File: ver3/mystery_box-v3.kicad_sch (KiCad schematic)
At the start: 31 parts, among them J10 Screw_Terminal_01x02, J11 Screw_Terminal_01x02, J12 Screw_Terminal_01x02, J13 Screw_Terminal_01x02, J14 Screw_Terminal_01x02, J15 Screw_Terminal_01x02, J16 Screw_Terminal_01x02, J17 Screw_Terminal_01x02, J18 Barrel_Jack_MountingPin, J20 rj45-CC-X2-Aliexpress, J8 Screw_Terminal_01x02, J9 Screw_Terminal_01x02, Q1 IRLZ44N, Q2 IRLZ44N, Q3 IRLZ44N, U2 MAX485E

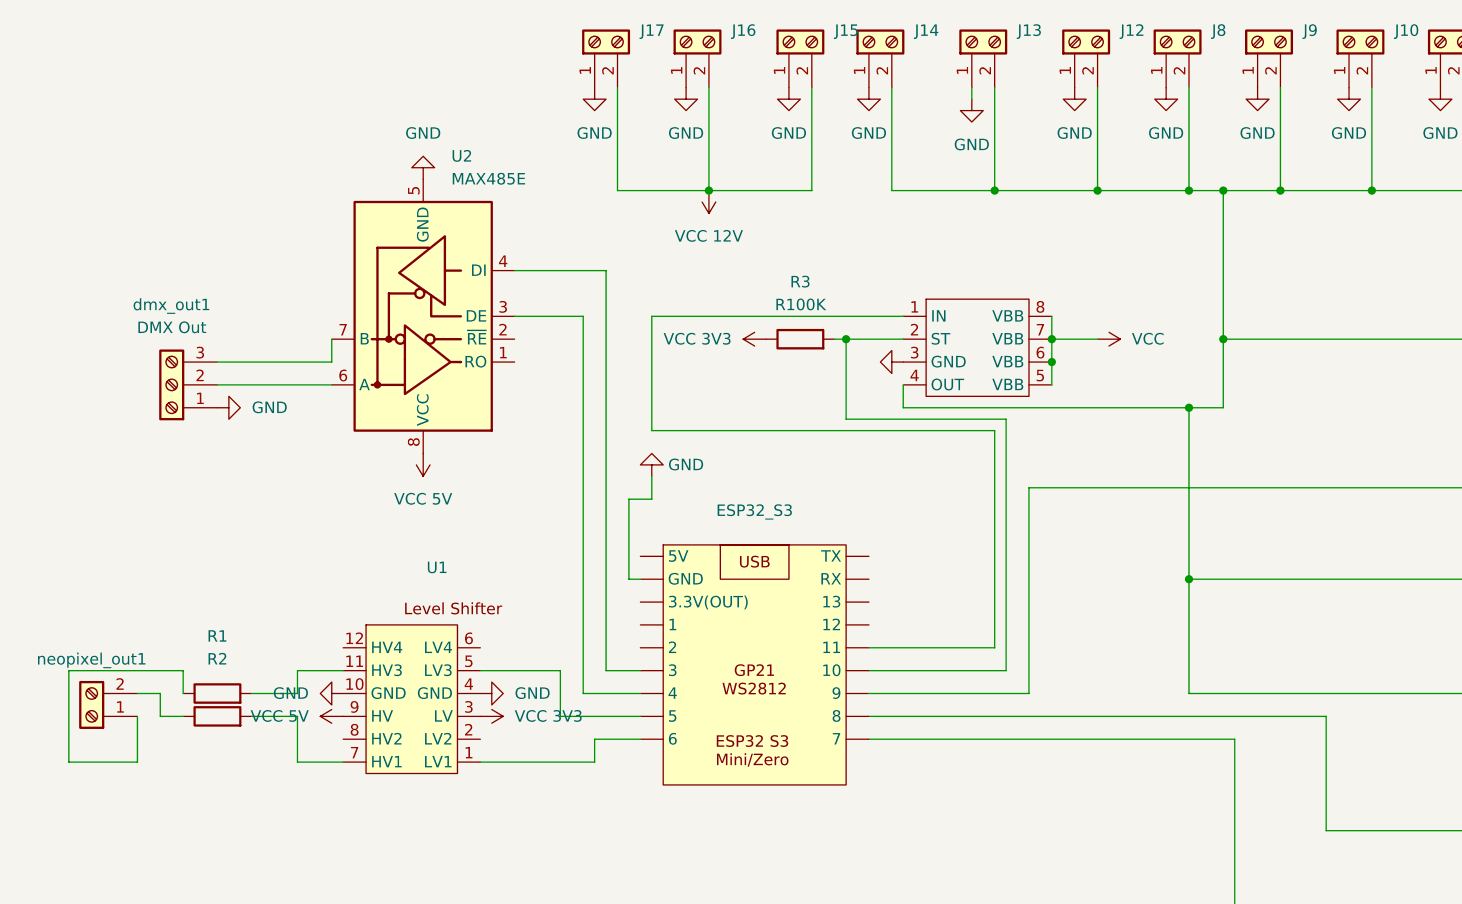
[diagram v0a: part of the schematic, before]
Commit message: final prototype v3
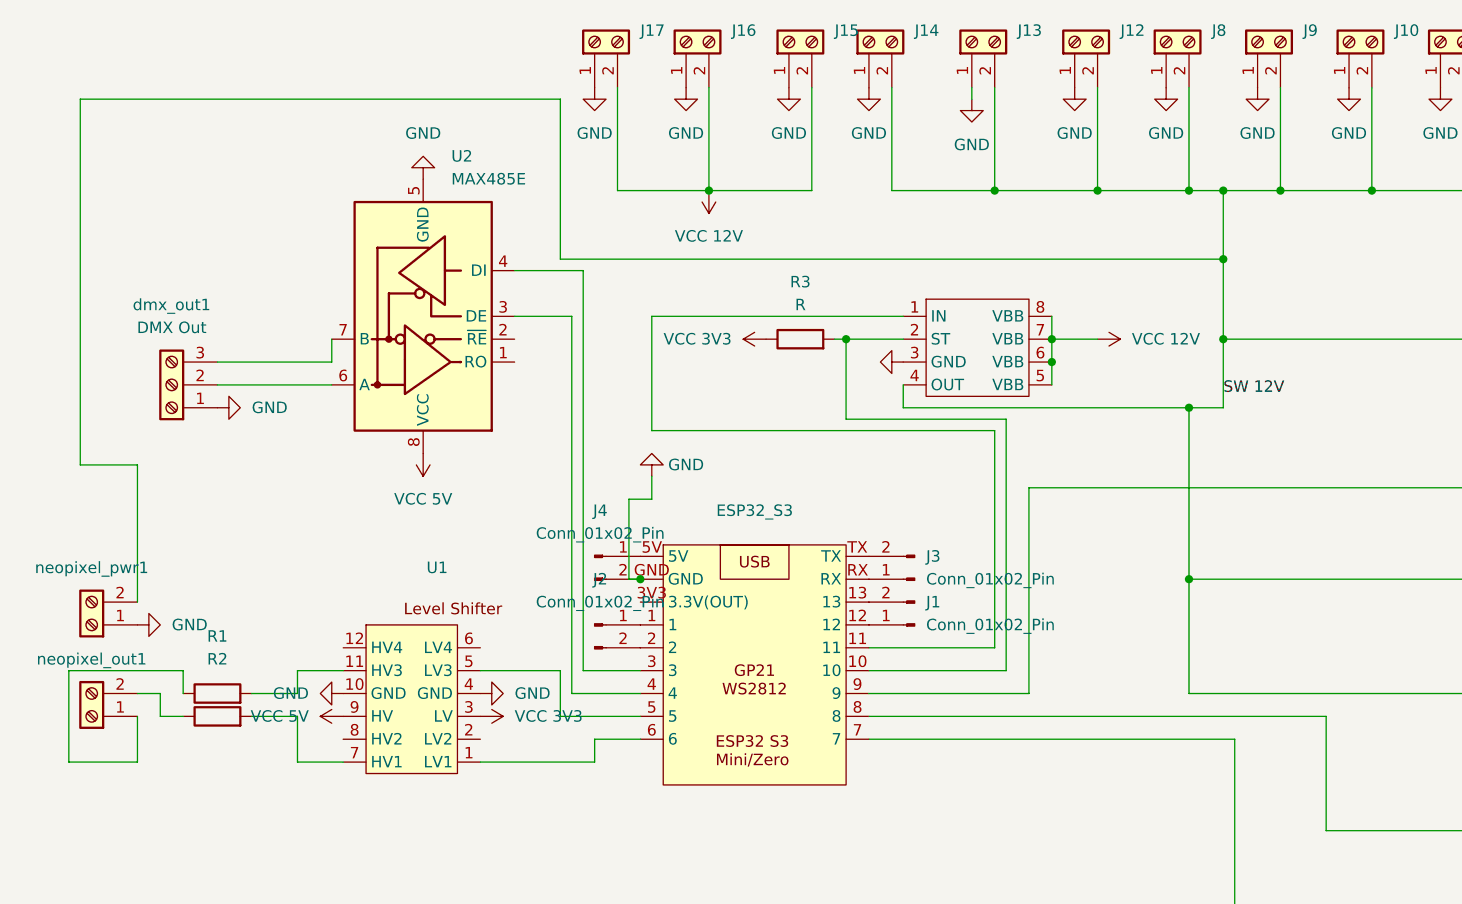
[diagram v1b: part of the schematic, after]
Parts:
- added J1, J2, J3, J4: Conn_01x02_Pin, Connector_PinHeader_1.00mm:PinHeader_1x02_P1.00mm_Vertical, symbol Connector:Conn_01x02_Pin
- added neopixel_pwr1: Screw_Terminal_01x02, TerminalBlock:TerminalBlock_MaiXu_MX126-5.0-02P_1x02_P5.00mm, symbol Connector:Screw_Terminal_01x02
- R3: value R100K -> R
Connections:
- net VCC is gone; now on net VCC 12V: U3.5 (VBB), U3.6 (VBB), U3.7 (VBB), U3.8 (VBB)
- net GND: now also ESP32_S3.GND, J4.2 (Pin_2), neopixel_pwr1.1 (Pin_1); no longer ESP32_S3. (7)
- net at Q1.1 (G): now also ESP32_S3.8; no longer ESP32_S3. (7)
- net at Q2.1 (G): now also ESP32_S3.7; no longer ESP32_S3. (7)
- net at Q3.1 (G): now also ESP32_S3.9; no longer ESP32_S3. (7)
- net at U3.1 (IN): now also ESP32_S3.11; no longer ESP32_S3. (7)
- net at R3.2, U3.2 (ST): now also ESP32_S3.10; no longer ESP32_S3. (7)
- net at U1.1 (LV1): now also ESP32_S3.6; no longer ESP32_S3. (7)
- net at U1.5 (LV3): now also ESP32_S3.5; no longer ESP32_S3. (7)
- net at U2.3 (DE): now also ESP32_S3.4; no longer ESP32_S3. (7)
- net at U2.4 (DI): now also ESP32_S3.3; no longer ESP32_S3. (7)
- net SW 12V: now reaches D1.1 (K), D2.1 (K), D3.1 (K), J10.2 (Pin_2), J11.2 (Pin_2), J12.2 (Pin_2), J13.2 (Pin_2), J14.2 (Pin_2), J8.2 (Pin_2), J9.2 (Pin_2), U3.4 (OUT), switched_output_01.1 (Pin_1), switched_output_02.1 (Pin_1), switched_output_03.1 (Pin_1)
- net SW 12V: now also neopixel_pwr1.2 (Pin_2)
- new net: ESP32_S3.1, J2.1 (Pin_1)
- new net: ESP32_S3.12, J1.1 (Pin_1)
- new net: ESP32_S3.13, J1.2 (Pin_2)
- new net: ESP32_S3.2, J2.2 (Pin_2)
- new net: ESP32_S3.5V, J4.1 (Pin_1)
- new net: ESP32_S3.RX, J3.1 (Pin_1)
- new net: ESP32_S3.TX, J3.2 (Pin_2)

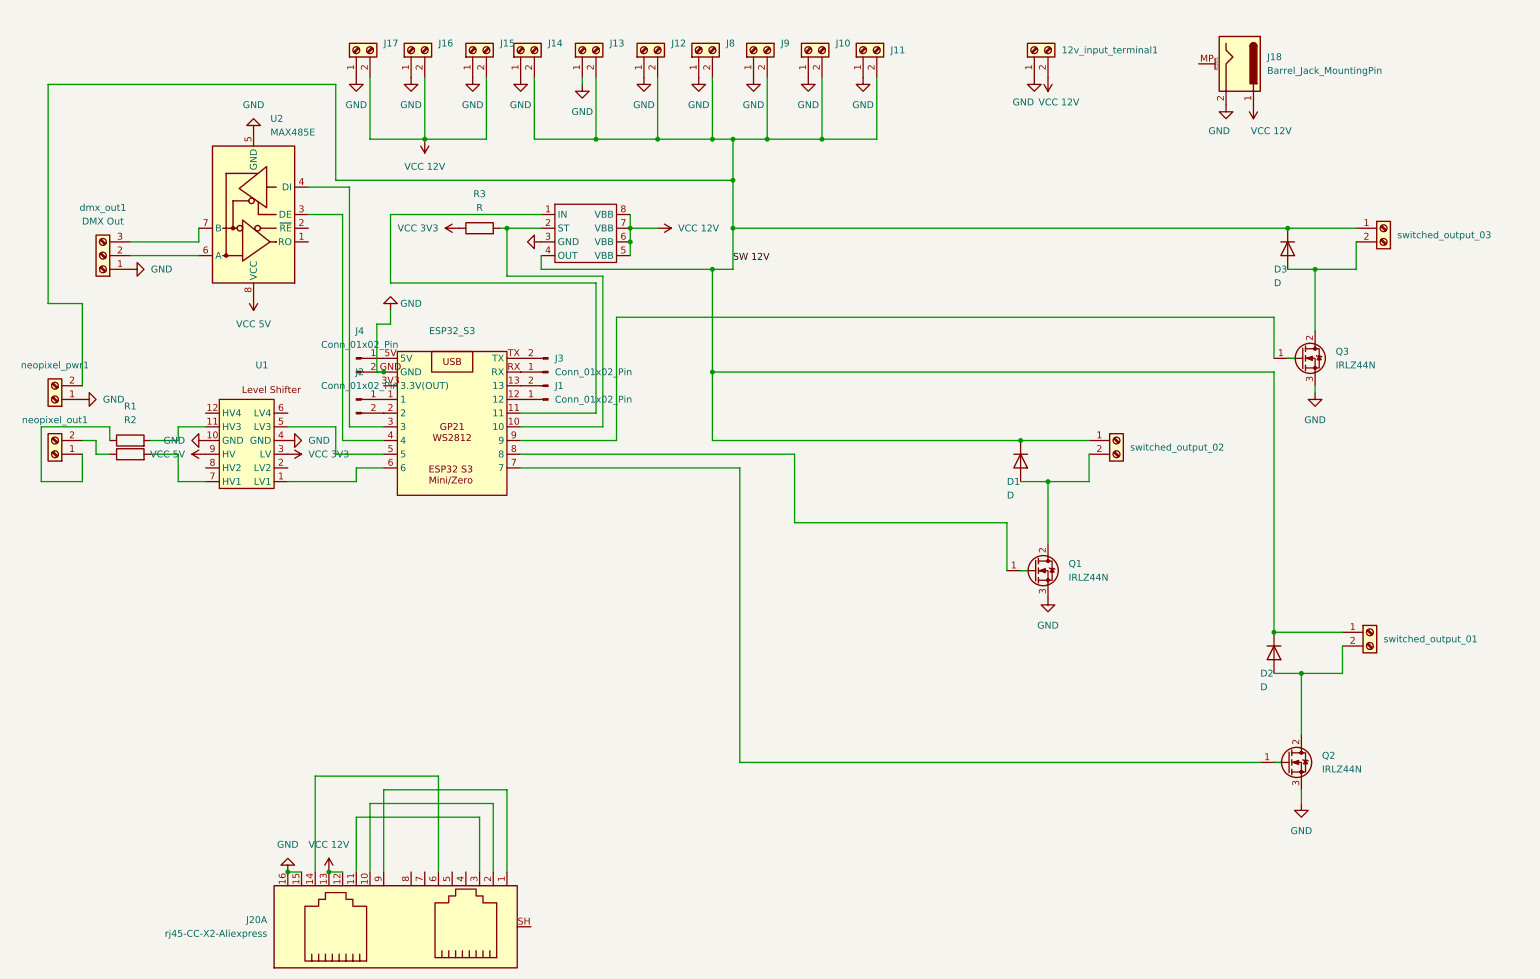
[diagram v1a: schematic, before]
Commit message: first edit of serious ver3
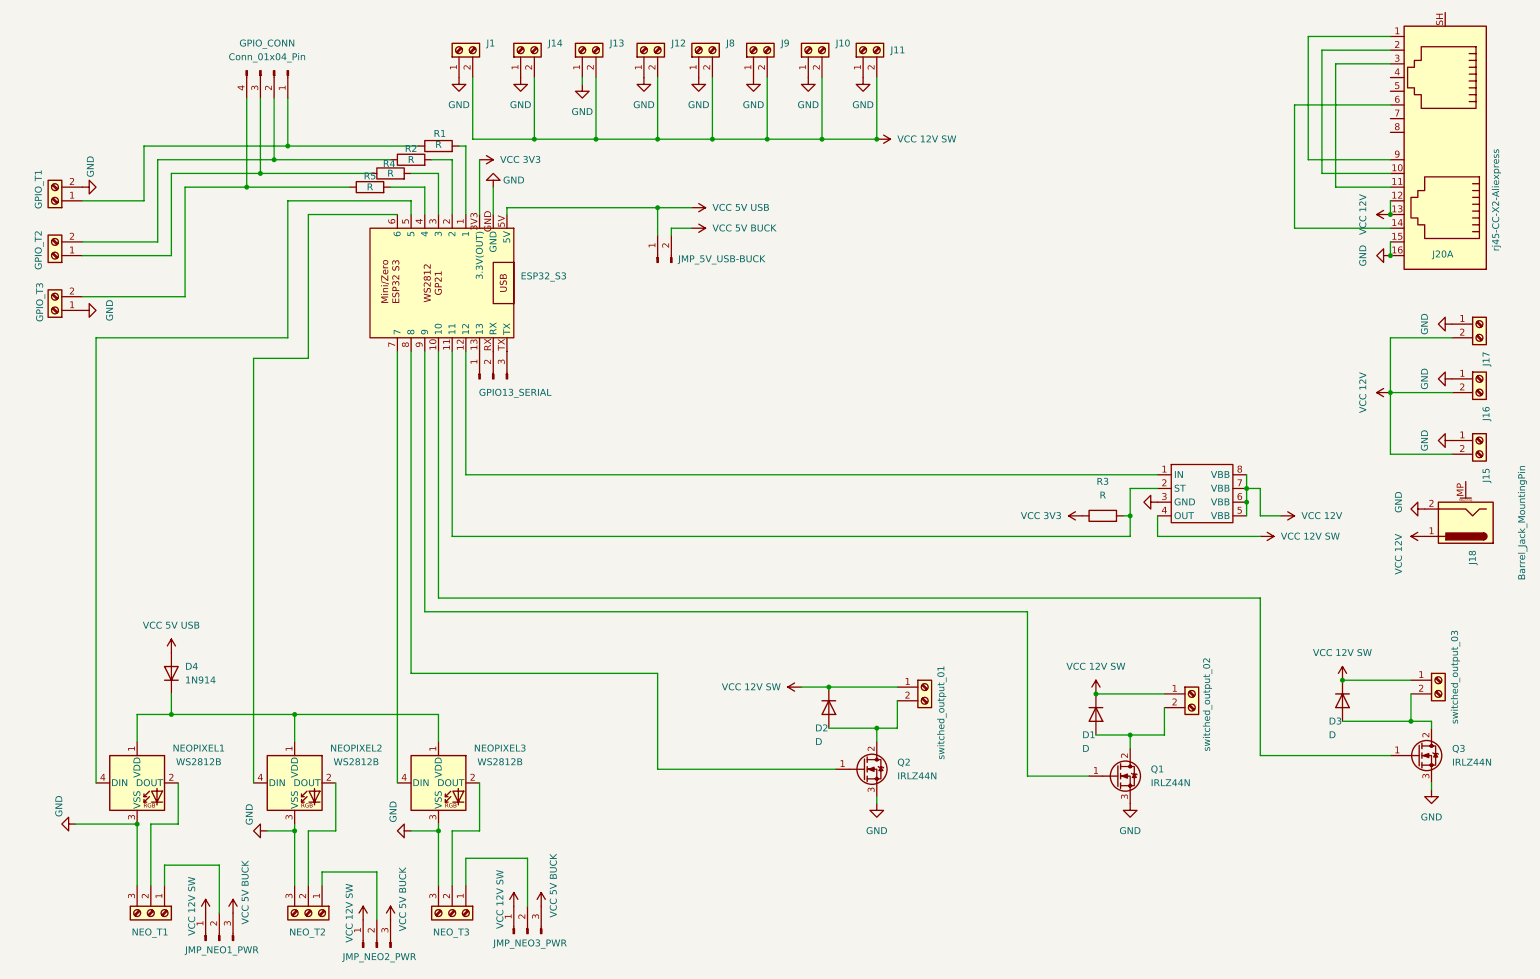
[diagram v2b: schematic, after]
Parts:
- removed 12v_input_terminal1, neopixel_out1, neopixel_pwr1: Screw_Terminal_01x02, TerminalBlock:TerminalBlock_MaiXu_MX126-5.0-02P_1x02_P5.00mm, symbol Connector:Screw_Terminal_01x02
- removed J1, J2, J3, J4: Conn_01x02_Pin, Connector_PinHeader_1.00mm:PinHeader_1x02_P1.00mm_Vertical, symbol Connector:Conn_01x02_Pin
- removed U1: ~, eigene_footprints:level_shifter, symbol eigene:levelshifter_2channel
- removed U2: MAX485E, eigene_footprints:max845 modul, symbol Interface_UART:MAX485E
- removed dmx_out1: DMX Out, TerminalBlock:TerminalBlock_MaiXu_MX126-5.0-03P_1x03_P5.00mm, symbol Connector:Screw_Terminal_01x03
- added D4: 1N914, Diode_THT:D_DO-35_SOD27_P7.62mm_Horizontal, symbol Diode:1N914
- added GPIO13_SERIAL, JMP_NEO1_PWR, JMP_NEO2_PWR, JMP_NEO3_PWR: Conn_01x03_Pin, symbol Connector:Conn_01x03_Pin
- added GPIO_CONN: Conn_01x04_Pin, symbol Connector:Conn_01x04_Pin
- added GPIO_T1, GPIO_T2, GPIO_T3, J1: Screw_Terminal_01x02, TerminalBlock:TerminalBlock_MaiXu_MX126-5.0-02P_1x02_P5.00mm, symbol Connector:Screw_Terminal_01x02
- added JMP_5V_USB-BUCK: Conn_01x02_Pin, symbol Connector:Conn_01x02_Pin
- added NEOPIXEL1, NEOPIXEL2, NEOPIXEL3: WS2812B, LED_SMD:LED_WS2812B_PLCC4_5.0x5.0mm_P3.2mm, symbol LED:WS2812B
- added NEO_T1, NEO_T2, NEO_T3: Screw_Terminal_01x03, symbol Connector:Screw_Terminal_01x03
- added R4, R5: R, symbol Device:R
- R1, R2: footprint Resistor_THT:R_Axial_DIN0207_L6.3mm_D2.5mm_P10.16mm_Horizontal -> (none)
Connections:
- net GND: now also GPIO_T1.2 (Pin_2), GPIO_T3.1 (Pin_1), J1.1 (Pin_1), NEOPIXEL1.3 (VSS), NEOPIXEL2.3 (VSS), NEOPIXEL3.3 (VSS), NEO_T1.3 (Pin_3), NEO_T2.3 (Pin_3), NEO_T3.3 (Pin_3)
- net VCC 3V3: now also ESP32_S3.3V3 (3.3V(OUT))
- net at R2.1: now also GPIO_CONN.2 (Pin_2), GPIO_T2.2 (Pin_2)
- net at R2.2: now also ESP32_S3.2
- net at ESP32_S3.1: now also R1.2
- net at R3.2, U3.2 (ST): now also ESP32_S3.11; no longer ESP32_S3.10
- net at U3.1 (IN): now also ESP32_S3.12; no longer ESP32_S3.11
- net at ESP32_S3.13: now also GPIO13_SERIAL.1 (Pin_1)
- net at ESP32_S3.3: now also R4.2
- net at ESP32_S3.4: now also R5.2
- net at ESP32_S3.5: now also NEOPIXEL1.4 (DIN)
- net VCC 5V USB: now reaches ESP32_S3.5V
- net VCC 5V USB: now also D4.2 (A), JMP_5V_USB-BUCK.1 (Pin_1)
- net at ESP32_S3.6: now also NEOPIXEL2.4 (DIN)
- net at ESP32_S3.7: now also NEOPIXEL3.4 (DIN); no longer Q2.1 (G)
- net at ESP32_S3.8: now also Q2.1 (G); no longer Q1.1 (G)
- net at Q3.1 (G): now also ESP32_S3.10; no longer ESP32_S3.9
- net at ESP32_S3.RX: now also GPIO13_SERIAL.2 (Pin_2)
- net at ESP32_S3.TX: now also GPIO13_SERIAL.3 (Pin_3)
- net at R1.1: now also GPIO_CONN.1 (Pin_1), GPIO_T1.1 (Pin_1)
- net SW 12V renamed VCC 12V SW
- net VCC 12V SW: now also J1.2 (Pin_2), JMP_NEO1_PWR.1 (Pin_1), JMP_NEO2_PWR.1 (Pin_1), JMP_NEO3_PWR.1 (Pin_1)
- new net: JMP_NEO3_PWR.2 (Pin_2), NEO_T3.1 (Pin_1)
- new net: JMP_NEO1_PWR.2 (Pin_2), NEO_T1.1 (Pin_1)
- new net: D4.1 (K), NEOPIXEL1.1 (VDD), NEOPIXEL2.1 (VDD), NEOPIXEL3.1 (VDD)
- new net: ESP32_S3.9, Q1.1 (G)
- new net: GPIO_CONN.3 (Pin_3), GPIO_T2.1 (Pin_1), R4.1
- new net: JMP_NEO2_PWR.2 (Pin_2), NEO_T2.1 (Pin_1)
- new net: NEOPIXEL2.2 (DOUT), NEO_T2.2 (Pin_2)
- new net: GPIO_CONN.4 (Pin_4), GPIO_T3.2 (Pin_2), R5.1
- new net: NEOPIXEL3.2 (DOUT), NEO_T3.2 (Pin_2)
- new net: NEOPIXEL1.2 (DOUT), NEO_T1.2 (Pin_2)
- new net VCC 5V BUCK: JMP_5V_USB-BUCK.2 (Pin_2), JMP_NEO1_PWR.3 (Pin_3), JMP_NEO2_PWR.3 (Pin_3), JMP_NEO3_PWR.3 (Pin_3)
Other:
- moved on the sheet: D1, D2, D3, ESP32_S3, J15, J16, J17, J18, J20A, Q1, Q2, Q3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
